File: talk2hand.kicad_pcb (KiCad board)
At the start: 2 copper layers, 14 x 18.5 mm, 4 parts, among them J1 USB_A, J2 USB_A

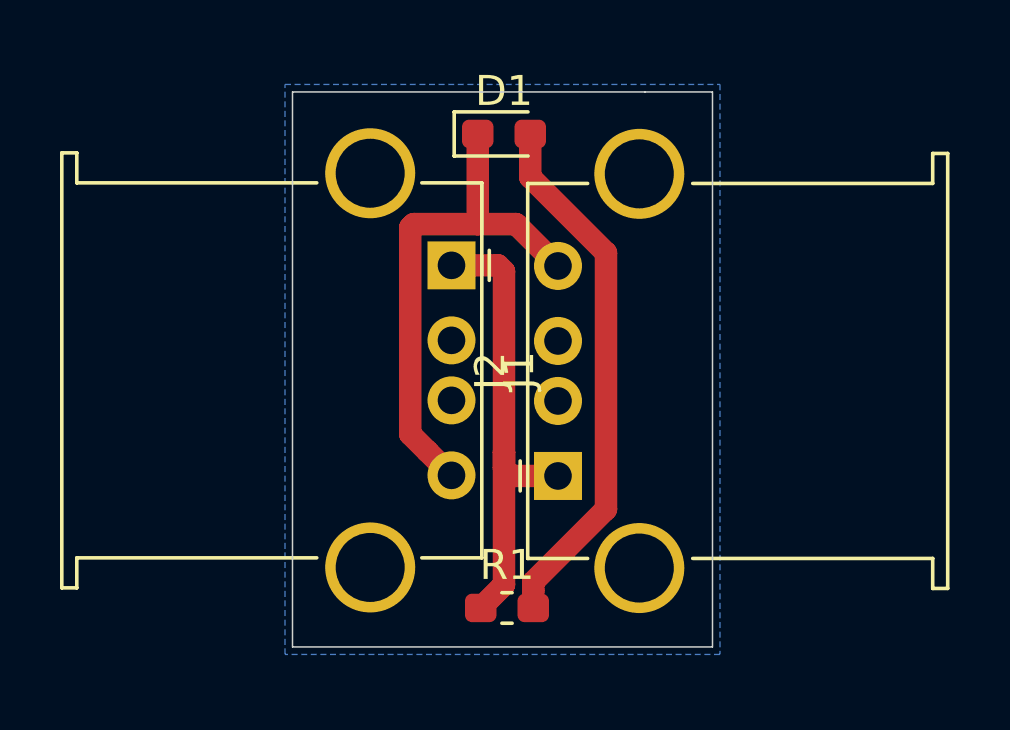
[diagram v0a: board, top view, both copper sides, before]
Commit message: PCB updates
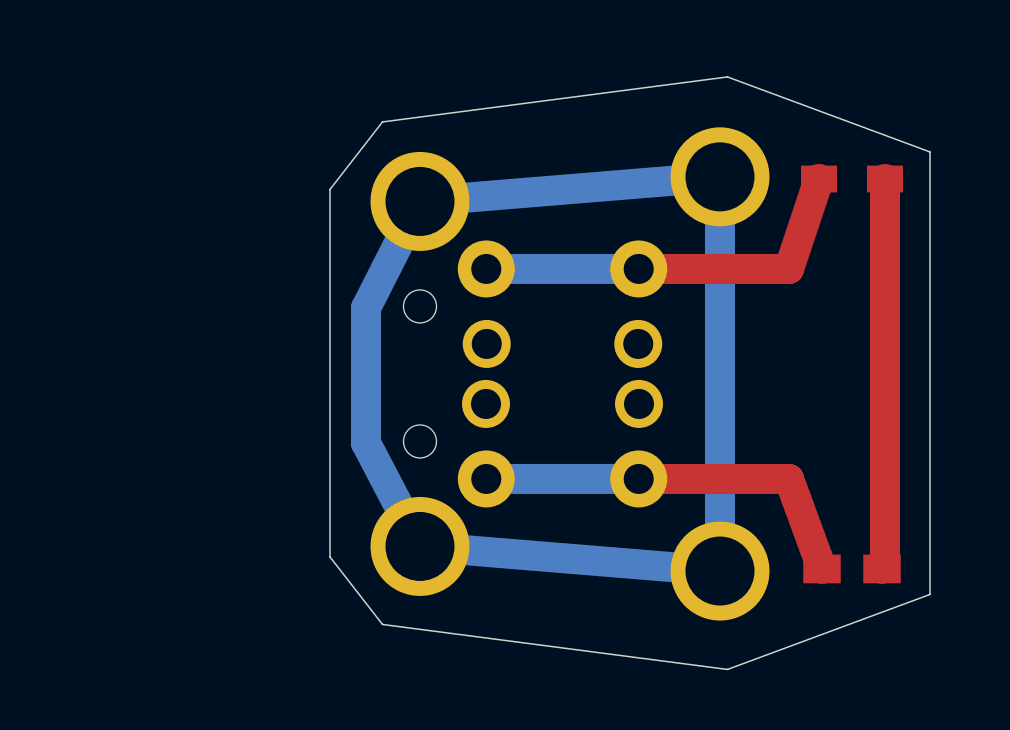
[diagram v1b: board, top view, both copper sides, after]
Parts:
- D1: footprint LED_SMD:LED_0603_1608Metric_Pad1.05x0.95mm_HandSolder -> BBS Components:LED_0603_HandSoldering
- J1: footprint Connector_USB:USB_A_Stewart_SS-52100-001_Horizontal -> BBS Components:USB_B_Male_Molex_0480370001
- J2: footprint Connector_USB:USB_A_Stewart_SS-52100-001_Horizontal -> BBS Components:USB_A_Female_Molex_0676432910; moved to B.Cu
- R1: footprint Resistor_SMD:R_0603_1608Metric_Pad1.05x0.95mm_HandSolder -> BBS Components:R_0603_HandSoldering_NoSilk
- moved D1 18.6 mm to (95.9, 91.4)
- moved R1 18.4 mm to (95.9, 78.4)
- moved J2 6.38 mm to (91.5, 84.9), turned to 270 degrees
- moved J1 3.77 mm to (81.5, 84.9)
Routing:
- net (no net): track 0.00 -> 45.7 mm
- net Net-(D1-Pad2): track 17.9 -> 13.0 mm
- net /gnd: track 17.4 -> 13.3 mm
- net /vbus: track 15.8 -> 13.3 mm
- removed copper zone on B.Cu, net /shield
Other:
- board size 14 x 18.5 mm -> 20 x 19.8 mm
